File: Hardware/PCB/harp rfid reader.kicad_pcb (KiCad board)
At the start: 4 copper layers, 45 x 26.5 mm, 65 parts, among them IC1 FT232RL, IC10 MC74VHC1GT125DBVT1G, IC2 NJM11100F1-TE2, IC3 ATxmega32A4U-A, IC4 MC74VHC1GT125DBVT1G, IC5 MC74VHC1GT125DBVT1G, J1 USB4105-GF-A, J2 282834-2, J3 NPPN051BFLD-RC, J4 NPPN071BFLC-RC, Q1 BC817-40W, Q2 NTF2955T1G, U2 TPD4E05U06DQA, X1 O 32,0-JT32C-A-K-3,3-LF

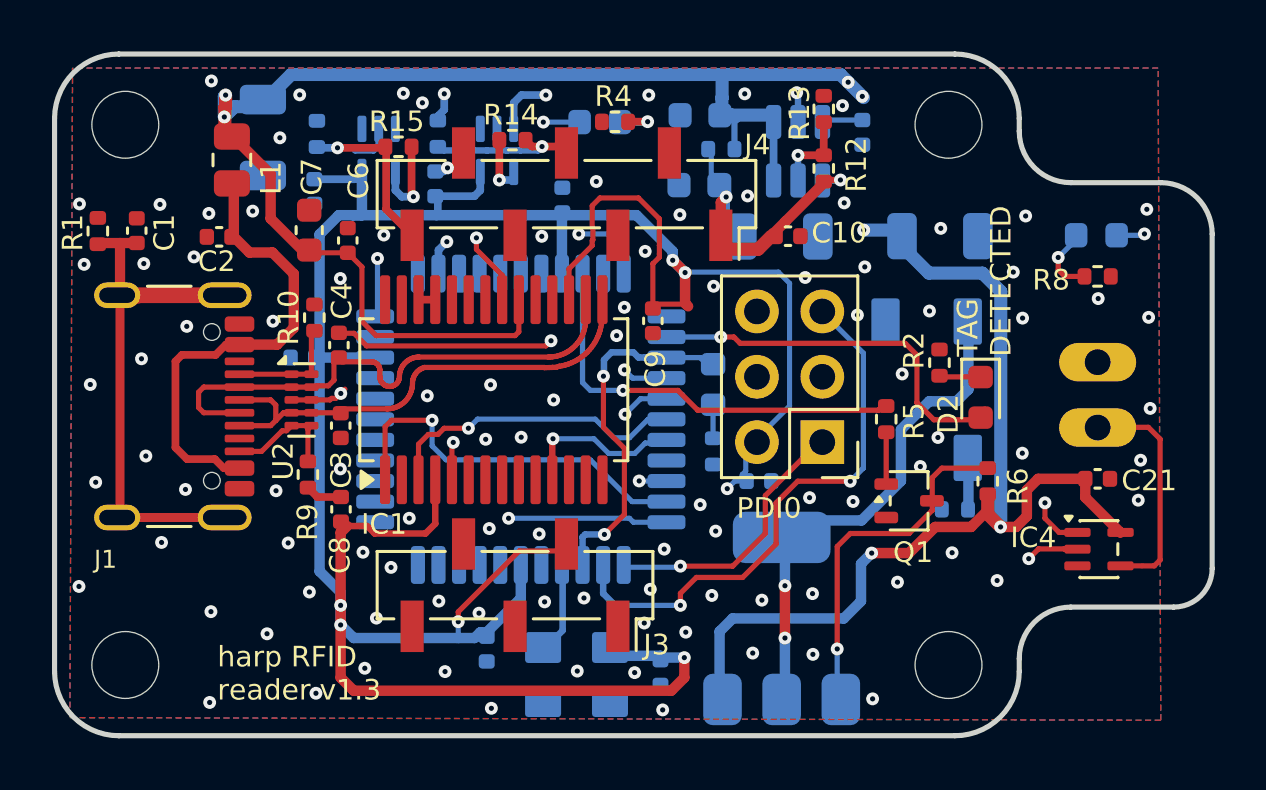
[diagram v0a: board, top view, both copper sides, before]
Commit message: dorrecção em ligação módulo RFID
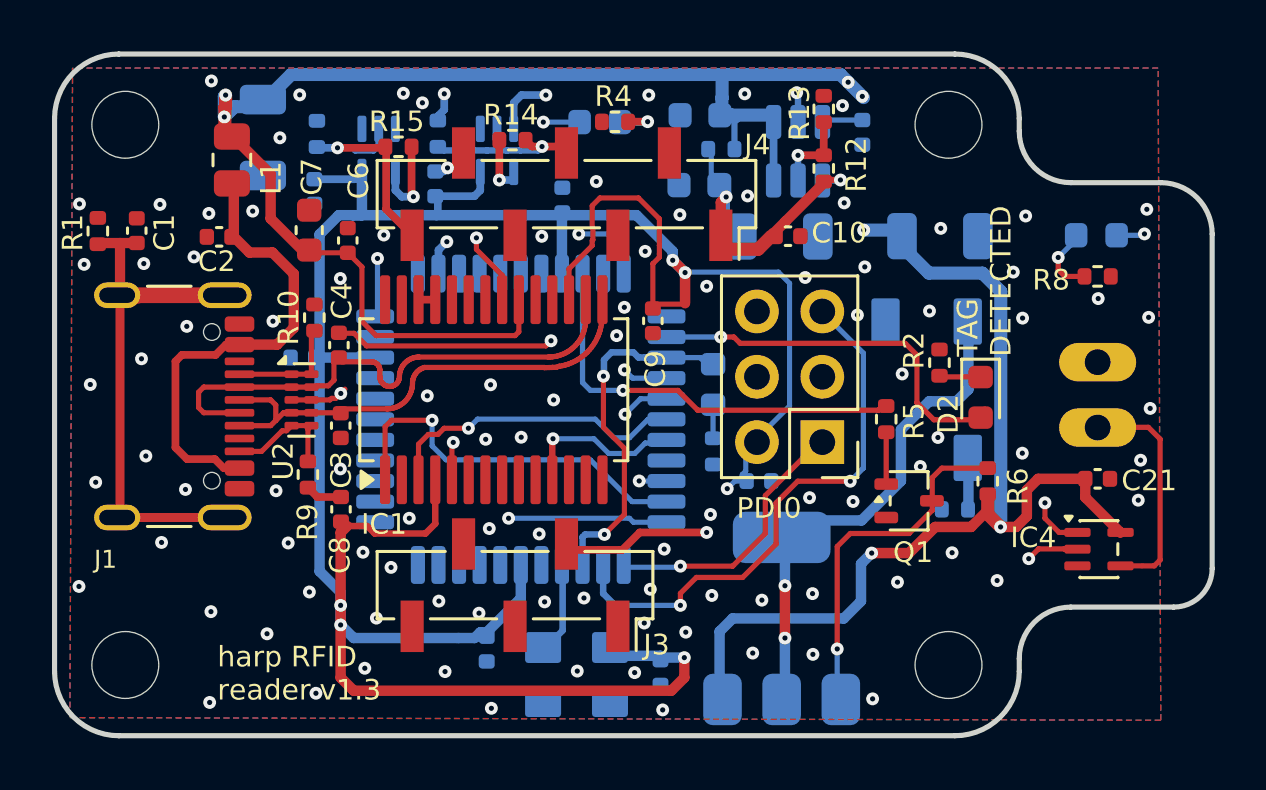
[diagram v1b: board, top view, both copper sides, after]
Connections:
- J3 pad 2: +3V3 -> VRFID
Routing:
- net VRFID: track 13.1 -> 33.4 mm, vias 2 -> 3
- net +3V3: track 119.5 -> 112.9 mm, vias 8 -> 7
- net GND: vias 104 -> 103
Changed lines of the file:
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@@
 			(size 2 0.9)
 			(layers "F.Cu" "F.Mask" "F.Paste")
-			(net "+3V3")
+			(net "VRFID")
 			(pinfunction "Pin_2_2")
 			(pintype "passive")
@@
 		(tags "resistor")
 		(property "Reference" "R3"
-			(at -0.87 -0.38 270)
+			(at -0.850799 -0.38 270)
 			(layer "B.SilkS")
 			(effects
@@
 	)
 	(via
-		(at 151.17 78.430801)
+		(at 150.9 78.430801)
 		(size 0.5)
 		(drill 0.2)
@@
 	)
 	(via
-		(at 151.25 87.949201)
-		(size 0.5)
-		(drill 0.2)
-		(layers "F.Cu" "B.Cu")
-		(net "GND")
-	)
-	(via
 		(at 127.15 86.049201)
 		(size 0.5)
@@
 	)
 	(via
-		(at 150.65 86.919201)
+		(at 151.049701 87.301171)
 		(size 0.5)
 		(drill 0.2)
@@
 	)
 	(segment
+		(start 147.621799 88.678201)
+		(end 145.679 88.678201)
+		(width 0.3)
+		(layer "F.Cu")
+		(net "VRFID")
+	)
+	(segment
+		(start 145.679 88.678201)
+		(end 145.45 88.449201)
+		(width 0.3)
+		(layer "F.Cu")
+		(net "VRFID")
+	)
+	(segment
+		(start 145.4655 88.465401)
+		(end 145.2115 88.719401)
+		(width 0.2032)
+		(layer "F.Cu")
+		(net "VRFID")
+	)
+	(segment
+		(start 150.9 88)
+		(end 148.3 88)
+		(width 0.3)
+		(layer "F.Cu")
+		(net "VRFID")
+	)
+	(segment
 		(start 153.4121 76.460801)
 		(end 153.4121 76.483801)
@@
 	)
 	(segment
+		(start 148.3 88)
+		(end 147.621799 88.678201)
+		(width 0.3)
+		(layer "F.Cu")
+		(net "VRFID")
+	)
+	(segment
 		(start 155.45 74.422901)
 		(end 155.45 74.359201)
@@
 	)
 	(via
+		(at 150.9 88)
+		(size 0.5)
+		(drill 0.2)
+		(layers "F.Cu" "B.Cu")
+		(free yes)
+		(net "VRFID")
+	)
+	(via
 		(at 151.6571 74.959801)
 		(size 0.5)
@@
 	)
 	(segment
+		(start 150.05 87.16773)
+		(end 150.401471 87.519201)
+		(width 0.3)
+		(layer "In2.Cu")
+		(net "VRFID")
+	)
+	(segment
+		(start 151.6571 74.959801)
+		(end 151.6571 78.79223)
+		(width 0.3)
+		(layer "In2.Cu")
+		(net "VRFID")
+	)
+	(segment
+		(start 150.401471 87.519201)
+		(end 150.419201 87.519201)
+		(width 0.3)
+		(layer "In2.Cu")
+		(net "VRFID")
+	)
+	(segment
+		(start 150 87.1)
+		(end 150.05 87.15)
+		(width 0.3)
+		(layer "In2.Cu")
+		(net "VRFID")
+	)
+	(segment
+		(start 150.419201 87.519201)
+		(end 150.9 88)
+		(width 0.3)
+		(layer "In2.Cu")
+		(net "VRFID")
+	)
+	(segment
+		(start 151.6571 78.79223)
+		(end 150 80.44933)
+		(width 0.3)
+		(layer "In2.Cu")
+		(net "VRFID")
+	)
+	(segment
+		(start 150 80.44933)
+		(end 150 87.1)
+		(width 0.3)
+		(layer "In2.Cu")
+		(net "VRFID")
+	)
+	(segment
+		(start 150.05 87.15)
+		(end 150.05 87.16773)
+		(width 0.3)
+		(layer "In2.Cu")
+		(net "VRFID")
+	)
+	(segment
 		(start 150.5525 83.249201)
 		(end 149.7815 82.478201)
@@
 	)
 	(segment
-		(start 145.2115 88.719401)
-		(end 143.6125 88.719401)
-		(width 0.2032)
-		(layer "F.Cu")
-		(net "+3V3")
-	)
-	(segment
 		(start 146.4783 76.627019)
 		(end 146.45 76.655319)
@@
 	)
 	(segment
-		(start 150.06 79.091101)
-		(end 150.1786 79.209701)
-		(width 0.4064)
-		(layer "F.Cu")
-		(net "+3V3")
-	)
-	(segment
 		(start 146.45 75.299201)
 		(end 146.45 76.143083)
@@
 	)
 	(segment
-		(start 145.4655 88.465401)
-		(end 145.2115 88.719401)
-		(width 0.2032)
-		(layer "F.Cu")
-		(net "+3V3")
-	)
-	(segment
 		(start 136.6711 91.596801)
 		(end 136.6711 90.834801)
@@
 	)
 	(segment
-		(start 150.1786 79.209701)
-		(end 150.0944 79.125501)
-		(width 0.2)
-		(layer "F.Cu")
-		(net "+3V3")
-	)
-	(segment
 		(start 146.4783 76.171383)
 		(end 146.4783 76.627019)
@@
 	)
 	(segment
-		(start 143.6125 88.719401)
-		(end 141.2431 91.088801)
-		(width 0.2032)
-		(layer "F.Cu")
-		(net "+3V3")
-	)
-	(segment
 		(start 148.8089 79.125501)
 		(end 148.8089 77.553661)
@@
 	)
 	(segment
-		(start 141.2431 91.088801)
-		(end 141.2431 91.469801)
-		(width 0.2032)
-		(layer "F.Cu")
-		(net "+3V3")
-	)
-	(segment
 		(start 136.6711 90.834801)
 		(end 136.6711 88.004901)
@@
 	)
 	(via
-		(at 141.2431 91.469801)
-		(size 0.5)
-		(drill 0.2)
-		(layers "F.Cu" "B.Cu")
-		(net "+3V3")
-	)
-	(via
 		(at 150.06 77.899201)
 		(size 0.5)
@@
 		(layer "B.Cu")
 		(net "+3V3")
-	)
-	(segment
-		(start 141.2431 91.469801)
-		(end 141.2431 92.104801)
-		(width 0.2032)
-		(layer "B.Cu")
-		(net "+3V3")
